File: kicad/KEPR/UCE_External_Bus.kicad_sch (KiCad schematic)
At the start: 6 parts, among them J10 Conn_02x40_Odd_Even, J13 PINHD_2x2_Male, J6 Conn_02x20_Odd_Even, J7 Conn_02x08_Odd_Even, J8 Conn_01x08_Pin, J9 Conn_02x40_Odd_Even

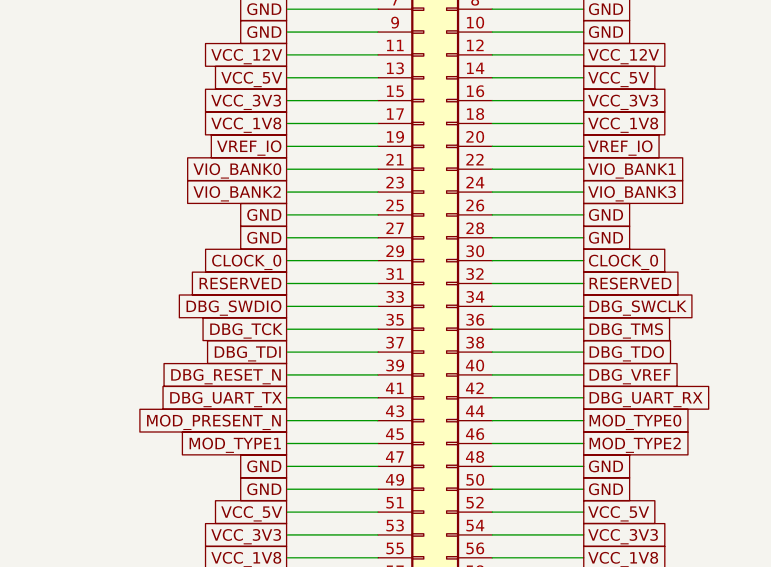
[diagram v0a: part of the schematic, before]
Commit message: mais ajustes de trilha.
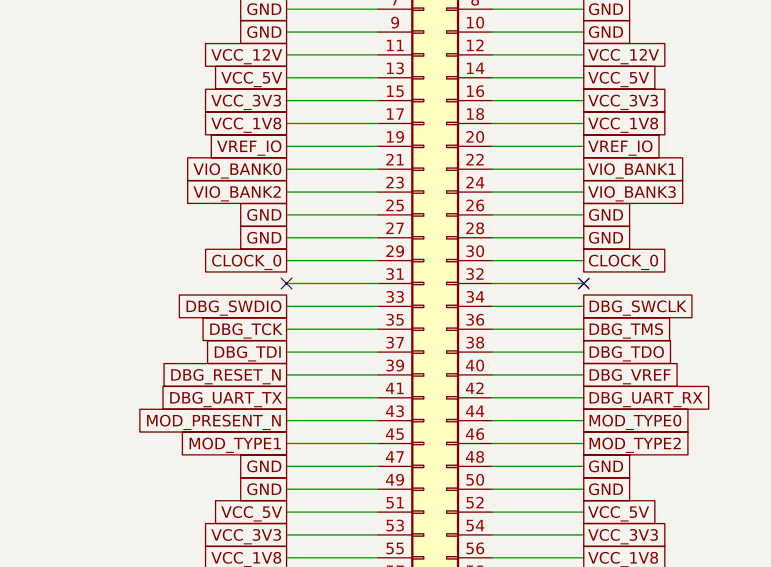
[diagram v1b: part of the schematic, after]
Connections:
- net RESERVED: no longer names the net of J10.31 (Pin_31)
- net RESERVED: no longer J10.32 (Pin_32)
- no-connect marks 31 -> 33
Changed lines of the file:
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@@
 	)
 	(no_connect
+		(at 254 121.92)
+	)
+	(no_connect
 		(at 287.02 177.8)
 	)
@@
 		(at 287.02 172.72)
 	)
+	(no_connect
+		(at 287.02 121.92)
+	)
 	(wire
 		(pts
@@
 		)
 	)
-	(global_label "RESERVED"
-		(shape passive)
-		(at 287.02 121.92 0)
-		(effects
-			(font
-				(size 1.27 1.27)
-			)
-			(justify left bottom)
-		)
-		(property "Intersheetrefs" "${INTERSHEET_REFS}"
-			(at 287.02 121.92 0)
-			(effects
-				(font
-					(size 1.27 1.27)
-				)
-				(hide yes)
-			)
-		)
-	)
 	(global_label "SPI1_SCK"
 		(shape passive)
@@
 			(effects
 				(font
-					(size 1.27 1.27)
-				)
-				(hide yes)
-			)
-		)
-	)
-	(global_label "RESERVED"
-		(shape passive)
-		(at 254 121.92 180)
-		(effects
-			(font
-				(size 1.27 1.27)
-			)
-			(justify right bottom)
-		)
-		(property "Intersheetrefs" "${INTERSHEET_REFS}"
-			(at 254 121.92 0)
-			(effects
-				(font
